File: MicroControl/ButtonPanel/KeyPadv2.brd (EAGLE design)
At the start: 59 x 109.8 mm, 27 parts, among them SW1 SW-12-12, SW10 SW-12-12, SW11 SW-12-12, SW12 SW-12-12, SW2 SW-12-12, SW3 SW-12-12, SW4 SW-12-12, SW5 SW-12-12, SW6 SW-12-12, SW7 SW-12-12, SW8 SW-12-12, SW9 SW-12-12

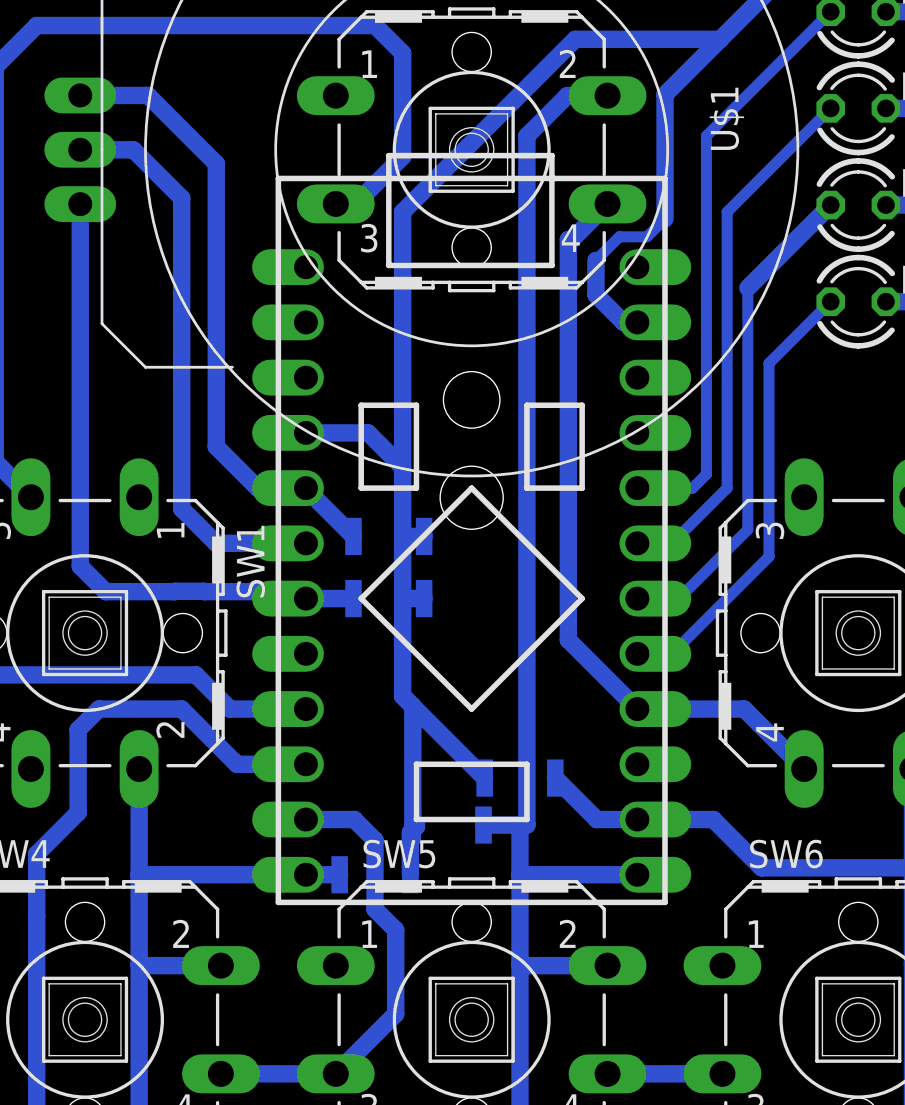
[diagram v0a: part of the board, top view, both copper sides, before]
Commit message: что-то ошло не так
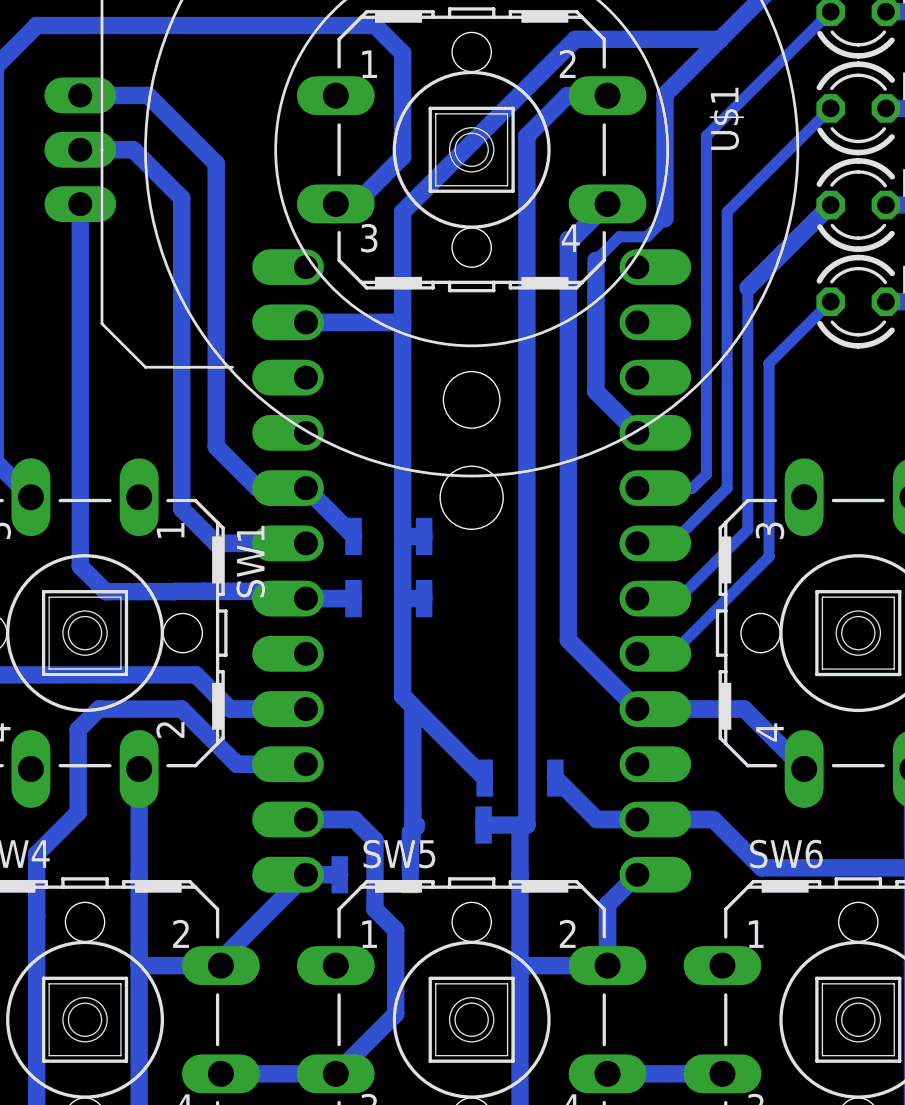
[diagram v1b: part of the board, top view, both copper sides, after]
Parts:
- flipped U$2 to the bottom
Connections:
- net COL1: now also U$2.10; no longer U$2.9
- net COL2: now also U$2.9; no longer U$2.10
- net COL3: now also U$2.8; no longer U$2.16
- net ENC-COM: now also U$2.20/A2; no longer U$2.3
- net ENC1: now also U$2.21/A3; no longer U$2.2
- net ENC2: now also U$2.19/A1; no longer U$2.4
- net MOD1: now also U$2.2; no longer U$2.21/A3
- net MOD2: now also U$2.3; no longer U$2.20/A2
- net MOD3: now also U$2.4; no longer U$2.19/A1
- net MOD4: now also U$2.5; no longer U$2.18/A0
- net ROW1: now also U$2.6; no longer U$2.15
- net ROW2: now also U$2.16; no longer U$2.8
- net ROW3: now also U$2.14; no longer U$2.7
- net ROW4: now also U$2.15; no longer U$2.6
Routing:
- net GND: track 113.3 -> 117.4 mm
- net COL1: track 62.9 -> 61.1 mm
- net COL2: track 95.3 -> 94.7 mm
